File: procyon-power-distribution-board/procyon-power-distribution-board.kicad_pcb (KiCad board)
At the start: 4 copper layers, 19 parts, among them Q1 BSS138, Q2 AO3401A, Q3 BSS138, Q4 AO3401A, Q5 BSS138, Q6 AO3401A, Q7 BSS138, Q8 AO3401A, U2 INA260

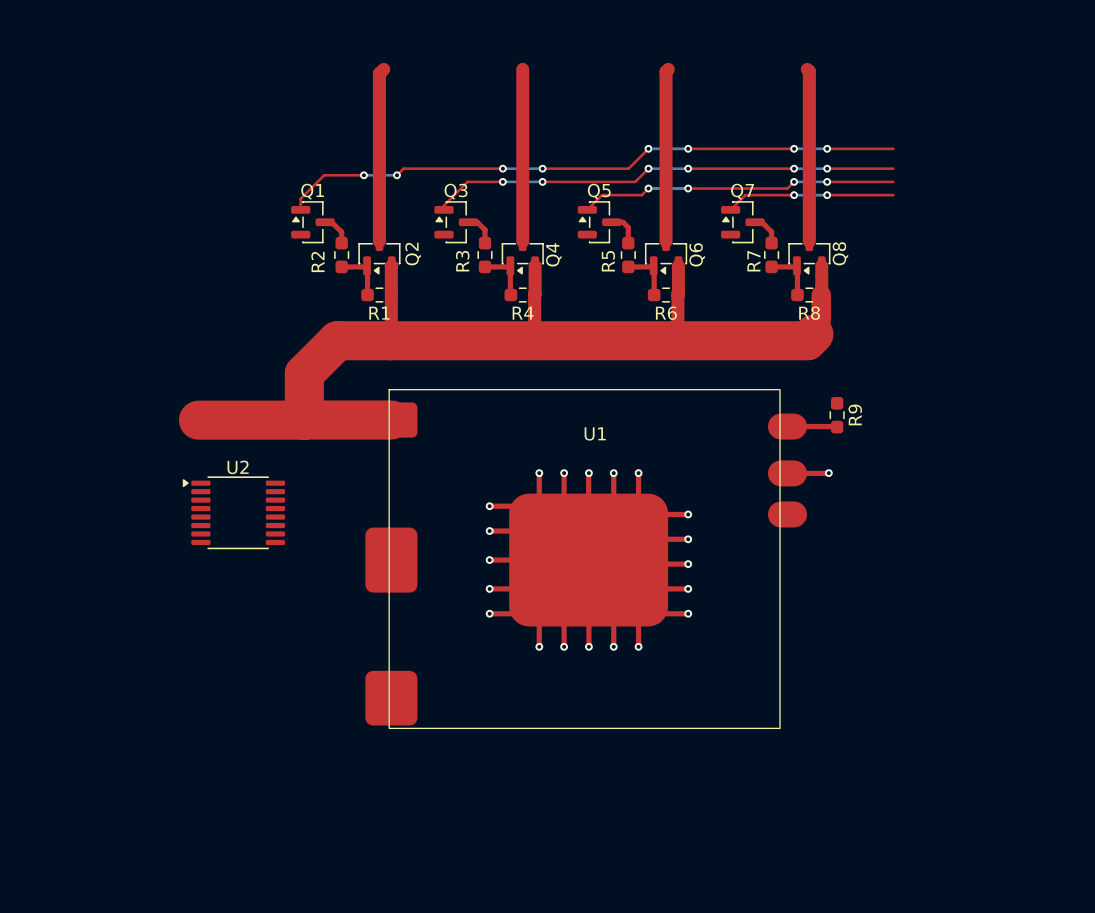
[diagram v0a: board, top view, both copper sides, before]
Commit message: Major changes, mostly finished, needs mounting holes and drc then finished.
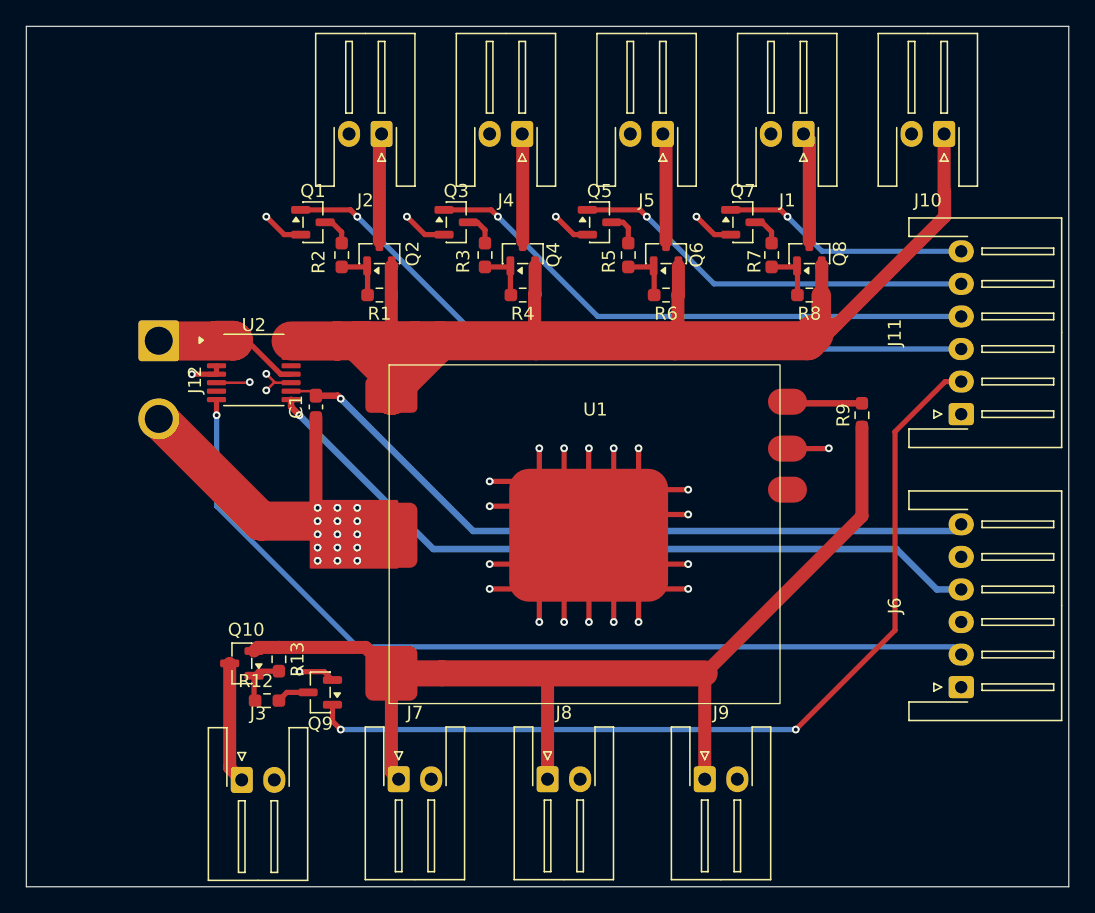
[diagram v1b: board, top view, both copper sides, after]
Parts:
- added C1: 100nF, Capacitor_SMD:C_0603_1608Metric_Pad1.08x0.95mm_HandSolder, F.Cu at (121.3, 83.8)
- added J1: BLDC_Pwr, Connector_JST:JST_XH_S2B-XH-A-1_1x02_P2.50mm_Horizontal, F.Cu at (158.7, 62.9)
- added J10: XTRA2_PWR, Connector_JST:JST_XH_S2B-XH-A-1_1x02_P2.50mm_Horizontal, F.Cu at (169.5, 62.9)
- added J11: Ctrl_Header, Connector_JST:JST_XH_S6B-XH-A-1_1x06_P2.50mm_Horizontal, F.Cu at (170.8, 84.4)
- added J12: BATT_IN, Connector_Wire:SolderWire-1.5sqmm_1x02_P6mm_D1.7mm_OD3mm, F.Cu at (109.2, 78.7)
- added J2: FPV1_Pwr, Connector_JST:JST_XH_S2B-XH-A-1_1x02_P2.50mm_Horizontal, F.Cu at (126.3, 62.9)
- added J3: BDC_Pwr, Connector_JST:JST_XH_S2B-XH-A-1_1x02_P2.50mm_Horizontal, F.Cu at (115.6, 112.5)
- added J4: FPV2_Pwr, Connector_JST:JST_XH_S2B-XH-A-1_1x02_P2.50mm_Horizontal, F.Cu at (137.1, 62.9)
- added J5: FPV3_Pwr, Connector_JST:JST_XH_S2B-XH-A-1_1x02_P2.50mm_Horizontal, F.Cu at (147.9, 62.9)
- added J6: INA260_Header, Connector_JST:JST_XH_S6B-XH-A-1_1x06_P2.50mm_Horizontal, F.Cu at (170.8, 105.3)
- added J7: FC_PWR, Connector_JST:JST_XH_S2B-XH-A-1_1x02_P2.50mm_Horizontal, F.Cu at (127.6, 112.4)
- added J8: Radio_PWR, Connector_JST:JST_XH_S2B-XH-A-1_1x02_P2.50mm_Horizontal, F.Cu at (139.1, 112.4)
- added J9: XTRA1_PWR, Connector_JST:JST_XH_S2B-XH-A-1_1x02_P2.50mm_Horizontal, F.Cu at (151.1, 112.4)
- added Q10: AO3401A, Package_TO_SOT_SMD:SOT-23, F.Cu at (115.6, 103.5)
- added Q9: BSS138, Package_TO_SOT_SMD:SOT-23, F.Cu at (121.6, 105.7)
- added R12: 220, Resistor_SMD:R_0603_1608Metric_Pad0.98x0.95mm_HandSolder, F.Cu at (117.5, 106.4)
- added R13: 10k, Resistor_SMD:R_0603_1608Metric_Pad0.98x0.95mm_HandSolder, F.Cu at (118.4, 103.2)
- R2, R3, R5, R7: value 100 -> 220
- moved U2 11.0 mm to (116.5, 81.0)
- moved R9 1.91 mm to (163.2, 84.5), turned to 90 degrees
- moved U1 1.91 mm to (142.2, 93.7)
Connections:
- Q2 pad 3: FPV_1_+ -> Net-(J2-Pin_1)
- Q4 pad 3: FPV_2_+ -> Net-(J4-Pin_1)
- Q6 pad 3: FPV_3_+ -> Net-(J5-Pin_1)
- Q8 pad 3: BLDC_1_+ -> Net-(J1-Pin_1)
- U2 pad 10: +5V -> +3V3
- U2 pad 8: INA_SDA -> Net-(J6-Pin_2)
- U2 pad 9: INA_SCL -> Net-(J6-Pin_4)
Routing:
- net +5V: track 0.00 -> 92.4 mm
- net Net-(J6-Pin_2): track 0.00 -> 70.1 mm, vias 0 -> 1
- net MCU_DC_0: track 0.00 -> 69.8 mm, vias 0 -> 2
- net Net-(J6-Pin_4): track 0.00 -> 57.8 mm, vias 0 -> 1
- net +3V3: track 0.00 -> 56.1 mm, vias 0 -> 1
- net GND: track 170.3 -> 209.3 mm, vias 21 -> 43
- net +BATT: track 80.4 -> 115.4 mm
- net FPV_1_+: track 13.3 -> 0.00 mm
- net FPV_3_+: track 13.3 -> 0.00 mm
- net BLDC_1_+: track 13.3 -> 0.00 mm
- net FPV_2_+: track 13.2 -> 0.00 mm
- net Net-(J3-Pin_1): track 0.00 -> 9.33 mm
- net Net-(J1-Pin_1): track 0.00 -> 8.44 mm
- net Net-(J5-Pin_1): track 0.00 -> 8.36 mm
- net Net-(J2-Pin_1): track 0.00 -> 8.32 mm
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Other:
- board outline added: 80 x 66 mm
